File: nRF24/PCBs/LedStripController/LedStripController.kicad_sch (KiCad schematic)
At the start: 19 parts, among them J1 Prog, J2 WS2812 1, J3 WS2812 2, J4 Bat 2, M1 TP4056, SW1 on/off, U1 NRF24L01, U2 ATtiny84, U3 MCP1700x-330

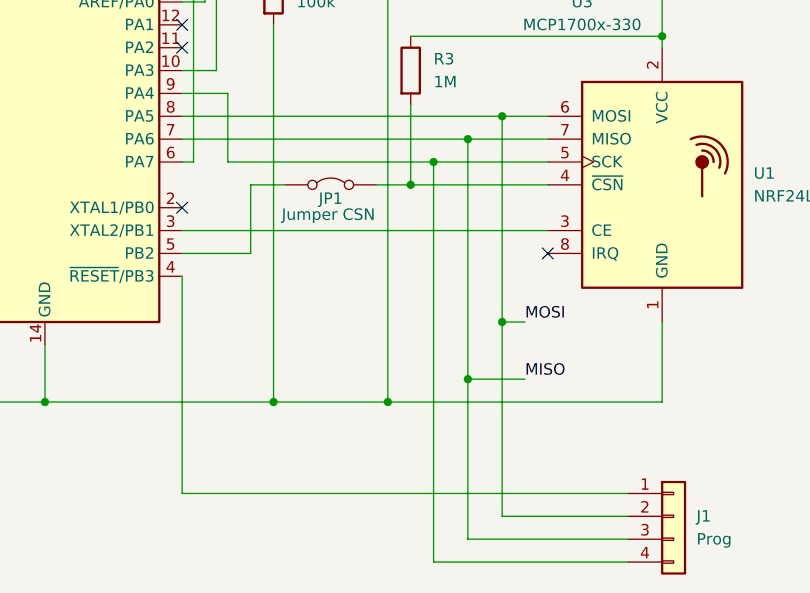
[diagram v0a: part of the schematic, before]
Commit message: nRF24 LED Strip Controller Debugging
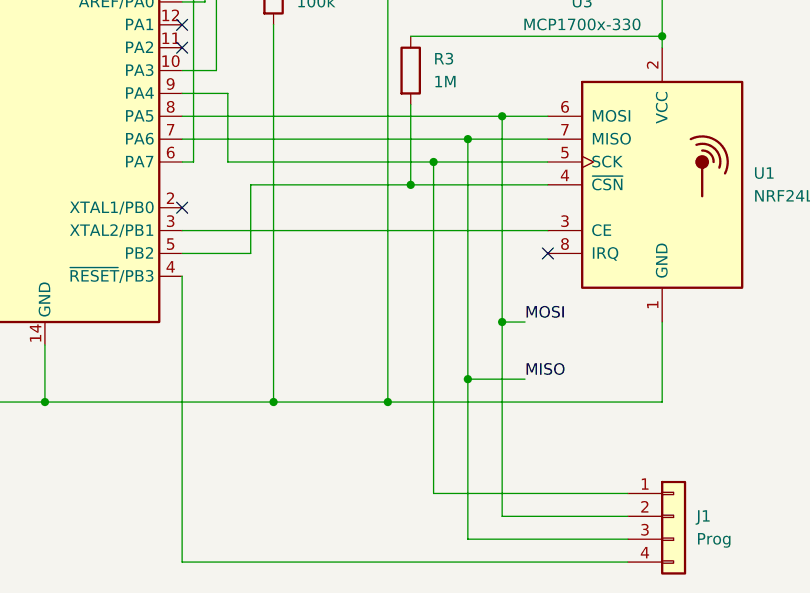
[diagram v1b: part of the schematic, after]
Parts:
- removed JP1: Jumper CSN, Connector_PinHeader_2.54mm:PinHeader_2x01_P2.54mm_Vertical, symbol Jumper:Jumper_2_Bridged
- M2: value ~ -> (none)
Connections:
- net at R3.2, U1.4 (~{CSN}): now also U2.5 (PB2)
- net at U1.5 (SCK), U2.9 (PA4): now also J1.1 (Pin_1); no longer J1.4 (Pin_4)
- net at U2.4 (~{RESET}/PB3): now also J1.4 (Pin_4); no longer J1.1 (Pin_1)
